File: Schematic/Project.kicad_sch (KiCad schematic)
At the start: 19 parts, among them J1 AC-IN, SW1 SW_Push, SW2 SW_Push, SW3 SW_Push, U1 MOC3021M

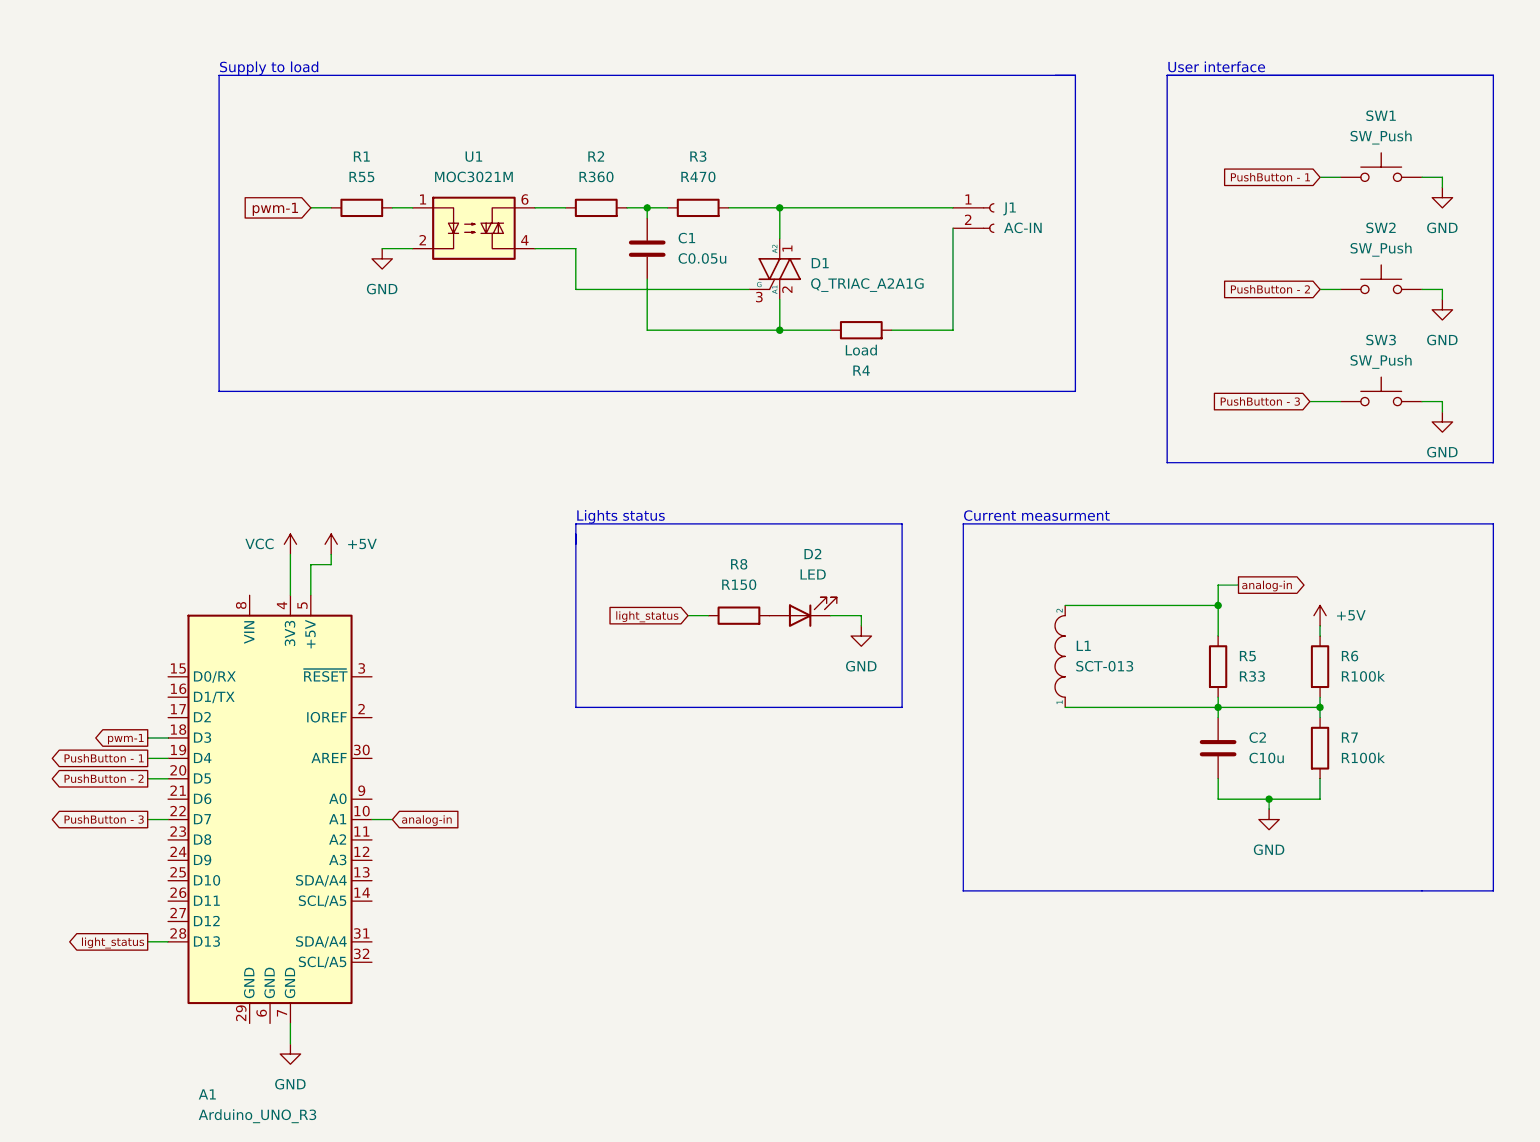
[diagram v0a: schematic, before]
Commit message: Fixed exit function
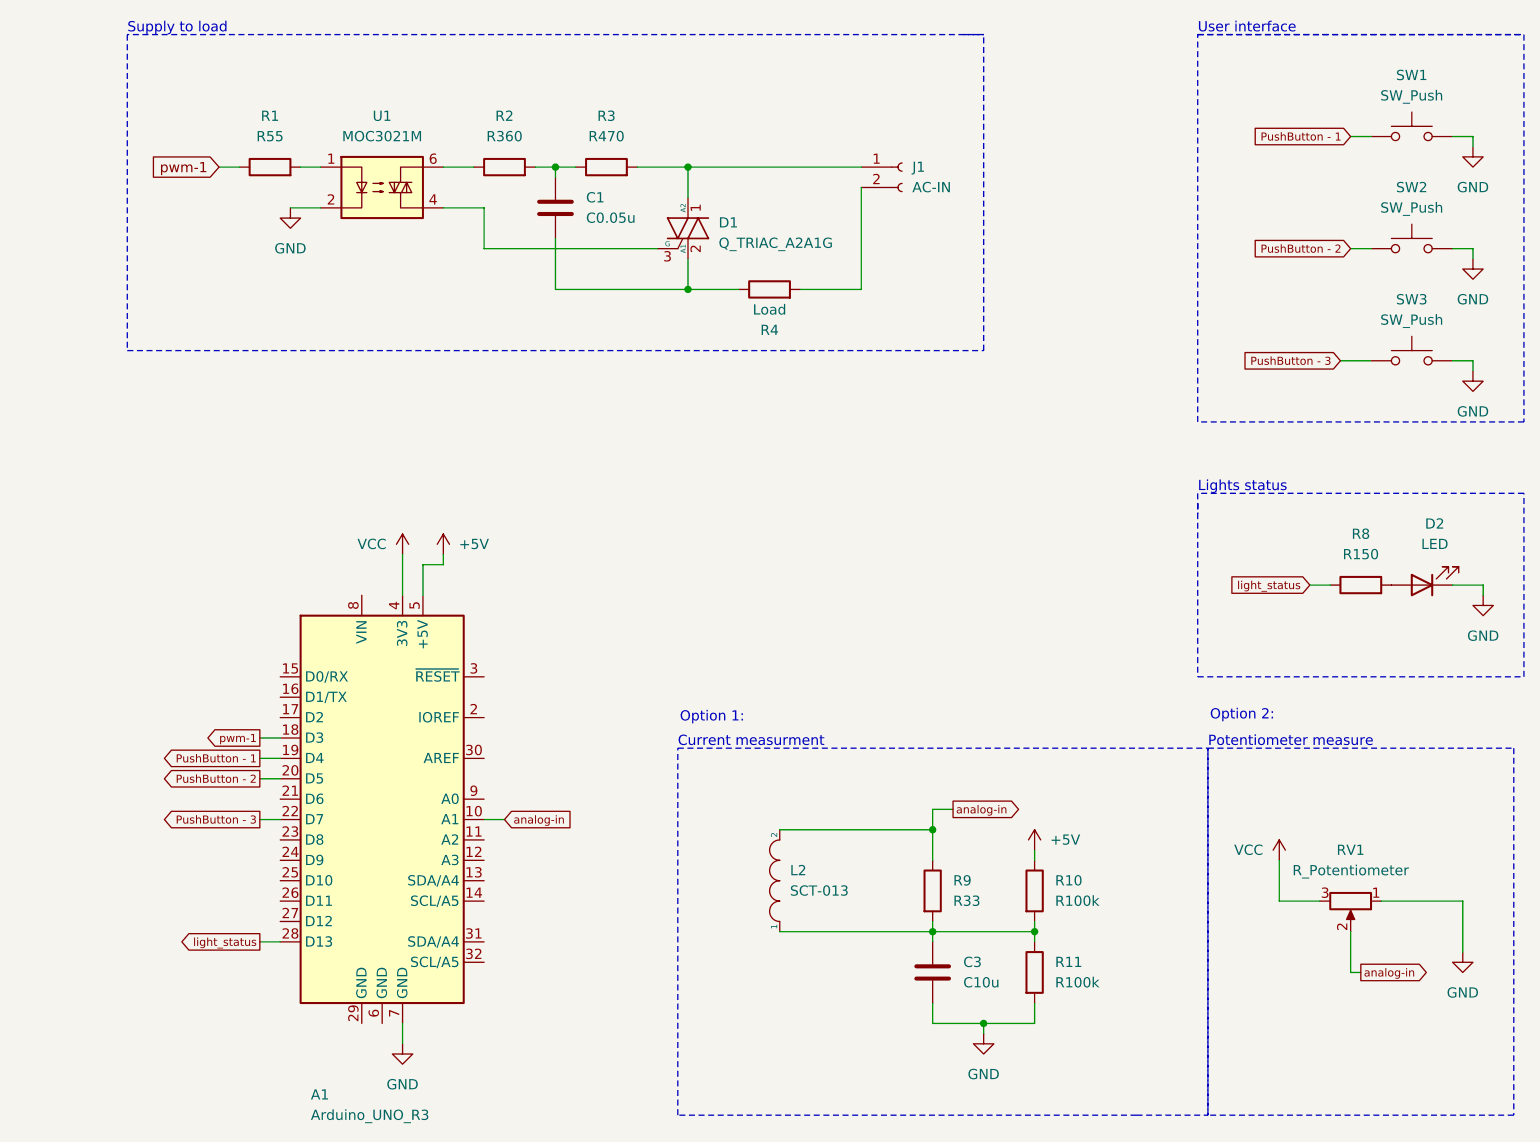
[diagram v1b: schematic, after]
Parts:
- removed C2: C10u, symbol Device:C
- removed L1: SCT-013, symbol pspice:INDUCTOR
- removed R5: R33, symbol Device:R
- removed R6, R7: R100k, symbol Device:R
- added C3: C10u, symbol Device:C
- added L2: SCT-013, symbol pspice:INDUCTOR
- added R10, R11: R100k, symbol Device:R
- added R9: R33, symbol Device:R
- added RV1: R_Potentiometer, symbol Device:R_Potentiometer
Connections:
- net +5V: now also R10.1
- net GND: now also C3.2, R11.2, RV1.1
- net VCC: now also RV1.3
- net analog-in: now also L2.2, R9.1, RV1.2
- new net: C3.1, L2.1, R10.2, R11.1, R9.2
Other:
- note added: "Option 1:"
- note added: "Option 2:"
- note added: "Potentiometer measure"
- moved on the sheet: A1, C1, D1, D2, J1, R1, R2, R3, R4, R8, SW1, SW2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
